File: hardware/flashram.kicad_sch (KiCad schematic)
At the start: 2 parts, among them U2 MT25QL256ABA1EW7-0SIT, U3 MT41K256M16TW-107:P

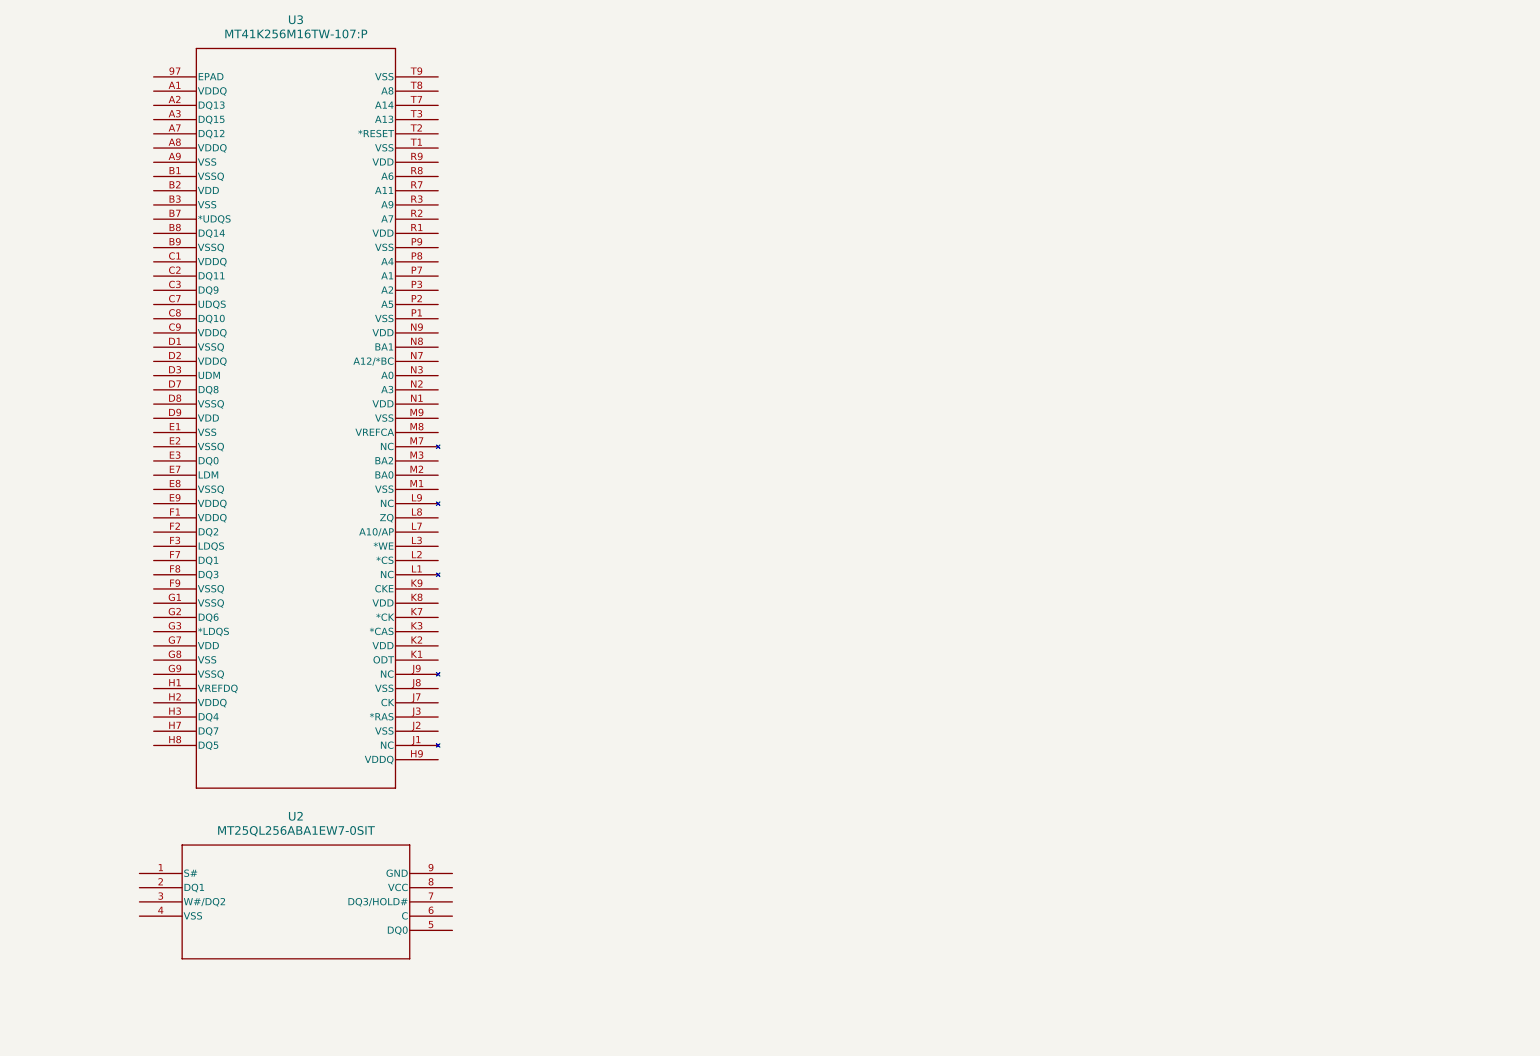
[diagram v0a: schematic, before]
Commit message: last commit for a while, i have to change the fpga and i dont have the time, money, or motivation to do that
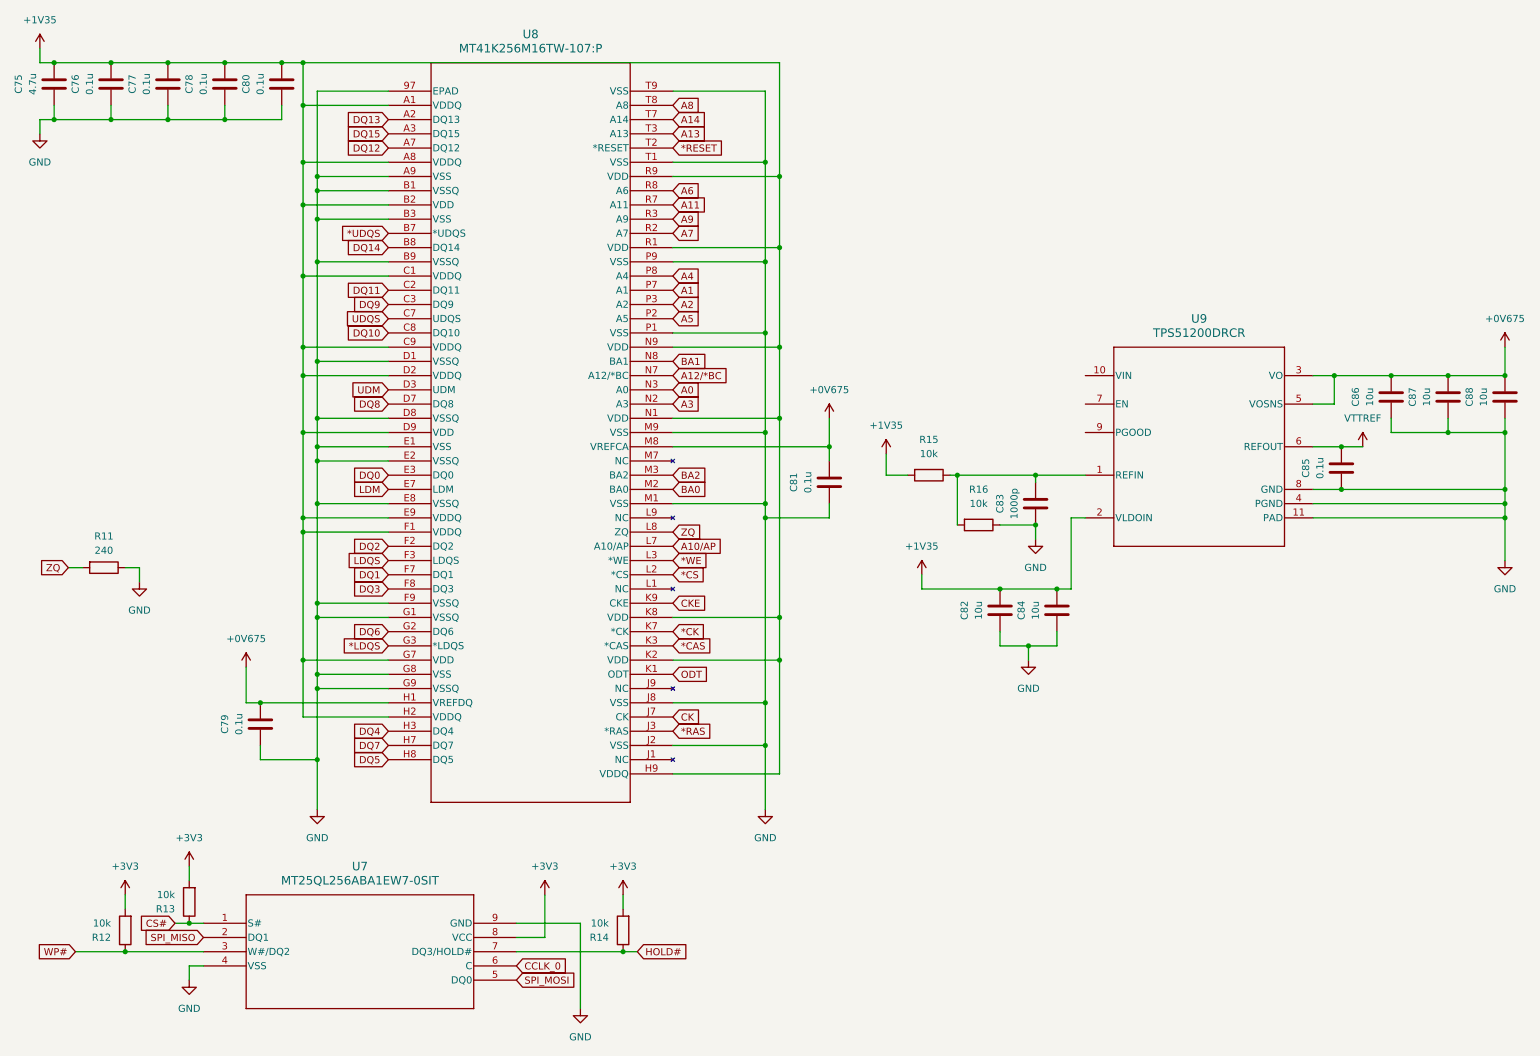
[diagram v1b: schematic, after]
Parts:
- added C75: 4.7u, symbol Device:C
- added C76, C77, C78, C79, C80, C81, C85: 0.1u, symbol Device:C
- added C82, C84, C86, C87, C88: 10u, symbol Device:C
- added C83: 1000p, symbol Device:C
- added R11: 240, symbol Device:R
- added R12, R13, R14, R15, R16: 10k, symbol Device:R
- added U9: TPS51200DRCR, DRC0010J, symbol arcticvideo:TPS51200DRCR
- renumbered U2 to U7, U3 to U8
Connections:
- net GND: now reaches U8.97 (EPAD)
- net GND: now also U7.4 (VSS), U7.9 (GND), U8.A9 (VSS), U8.B1 (VSSQ), U8.B3 (VSS), U8.B9 (VSSQ), U8.D1 (VSSQ), U8.D8 (VSSQ), U8.E1 (VSS), U8.E2 (VSSQ), U8.E8 (VSSQ), U8.F9 (VSSQ), U8.G1 (VSSQ), U8.G8 (VSS), U8.G9 (VSSQ), U8.J2 (VSS), U8.J8 (VSS), U8.M1 (VSS), U8.M9 (VSS), U8.P1 (VSS), U8.P9 (VSS), U8.T1 (VSS), U8.T9 (VSS), C75.1, C76.1, C77.1, C78.1, C79.1, C80.1, C81.1, C82.1, C83.1, C84.1, C85.1, C86.1, C87.1, C88.1, R11.1, R16.1, U9.11 (PAD), U9.4 (PGND), U9.8 (GND)
- net +1V35: now reaches U8.A1 (VDDQ)
- net +1V35: now also U8.A8 (VDDQ), U8.B2 (VDD), U8.C1 (VDDQ), U8.C9 (VDDQ), U8.D2 (VDDQ), U8.D9 (VDD), U8.E9 (VDDQ), U8.F1 (VDDQ), U8.G7 (VDD), U8.H2 (VDDQ), U8.H9 (VDDQ), U8.K2 (VDD), U8.K8 (VDD), U8.N1 (VDD), U8.N9 (VDD), U8.R1 (VDD), U8.R9 (VDD), C75.2, C76.2, C77.2, C78.2, C80.2, C82.2, C84.2, R15.2, U9.2 (VLDOIN)
- net DQ13: now reaches U8.A2 (DQ13)
- net DQ15: now reaches U8.A3 (DQ15)
- net DQ12: now reaches U8.A7 (DQ12)
- net *UDQS: now reaches U8.B7 (*UDQS)
- net DQ14: now reaches U8.B8 (DQ14)
- net DQ11: now reaches U8.C2 (DQ11)
- net DQ9: now reaches U8.C3 (DQ9)
- net UDQS: now reaches U8.C7 (UDQS)
- net DQ10: now reaches U8.C8 (DQ10)
- net UDM: now reaches U8.D3 (UDM)
- net DQ8: now reaches U8.D7 (DQ8)
- net DQ0: now reaches U8.E3 (DQ0)
- net LDM: now reaches U8.E7 (LDM)
- net DQ2: now reaches U8.F2 (DQ2)
- net LDQS: now reaches U8.F3 (LDQS)
- net DQ1: now reaches U8.F7 (DQ1)
- net DQ3: now reaches U8.F8 (DQ3)
- net DQ6: now reaches U8.G2 (DQ6)
- net *LDQS: now reaches U8.G3 (*LDQS)
- net +0V675: now reaches U8.H1 (VREFDQ)
- net +0V675: now also U8.M8 (VREFCA), C79.2, C81.2, C86.2, C87.2, C88.2, U9.3 (VO), U9.5 (VOSNS)
- net DQ4: now reaches U8.H3 (DQ4)
- net DQ7: now reaches U8.H7 (DQ7)
- net DQ5: now reaches U8.H8 (DQ5)
- net *RAS: now reaches U8.J3 (*RAS)
- net CK: now reaches U8.J7 (CK)
- net ODT: now reaches U8.K1 (ODT)
- net *CAS: now reaches U8.K3 (*CAS)
- net *CK: now reaches U8.K7 (*CK)
- net CKE: now reaches U8.K9 (CKE)
- net *CS: now reaches U8.L2 (*CS)
- net *WE: now reaches U8.L3 (*WE)
- net A10/AP: now reaches U8.L7 (A10/AP)
- net ZQ: now reaches U8.L8 (ZQ)
- net ZQ: now also R11.2
- net BA0: now reaches U8.M2 (BA0)
- net BA2: now reaches U8.M3 (BA2)
- net A3: now reaches U8.N2 (A3)
- net A0: now reaches U8.N3 (A0)
- net A12/*BC: now reaches U8.N7 (A12/*BC)
- net BA1: now reaches U8.N8 (BA1)
- net A5: now reaches U8.P2 (A5)
- net A2: now reaches U8.P3 (A2)
- net A1: now reaches U8.P7 (A1)
- net A4: now reaches U8.P8 (A4)
- net A7: now reaches U8.R2 (A7)
- net A9: now reaches U8.R3 (A9)
- net A11: now reaches U8.R7 (A11)
- net A6: now reaches U8.R8 (A6)
- net *RESET: now reaches U8.T2 (*RESET)
- net A13: now reaches U8.T3 (A13)
- net A14: now reaches U8.T7 (A14)
- net A8: now reaches U8.T8 (A8)
- net CS#: now reaches U7.1 (S#)
- net CS#: now also R13.1
- net SPI_MISO: now reaches U7.2 (DQ1)
- net WP#: now reaches U7.3 (W#/DQ2)
- net WP#: now also R12.1
- net SPI_MOSI: now reaches U7.5 (DQ0)
- net CCLK_0: now reaches U7.6 (C)
- net HOLD#: now reaches U7.7 (DQ3/HOLD#)
- net HOLD#: now also R14.1
- net +3V3: now reaches U7.8 (VCC)
- net +3V3: now also R12.2, R13.2, R14.2
- new net: C83.2, R15.1, R16.2, U9.1 (REFIN)
- new net VTTREF: C85.2, U9.6 (REFOUT)
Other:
- moved on the sheet: U7, U8
